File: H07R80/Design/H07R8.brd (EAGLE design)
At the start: 60 x 34.6 mm, 17 parts, among them P2 HEXABIT_X2_P1_P5_EDIT_POWER_P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, U1 STM32G0B1CEU6N, X1 XTALL_CSTCE8M00G52

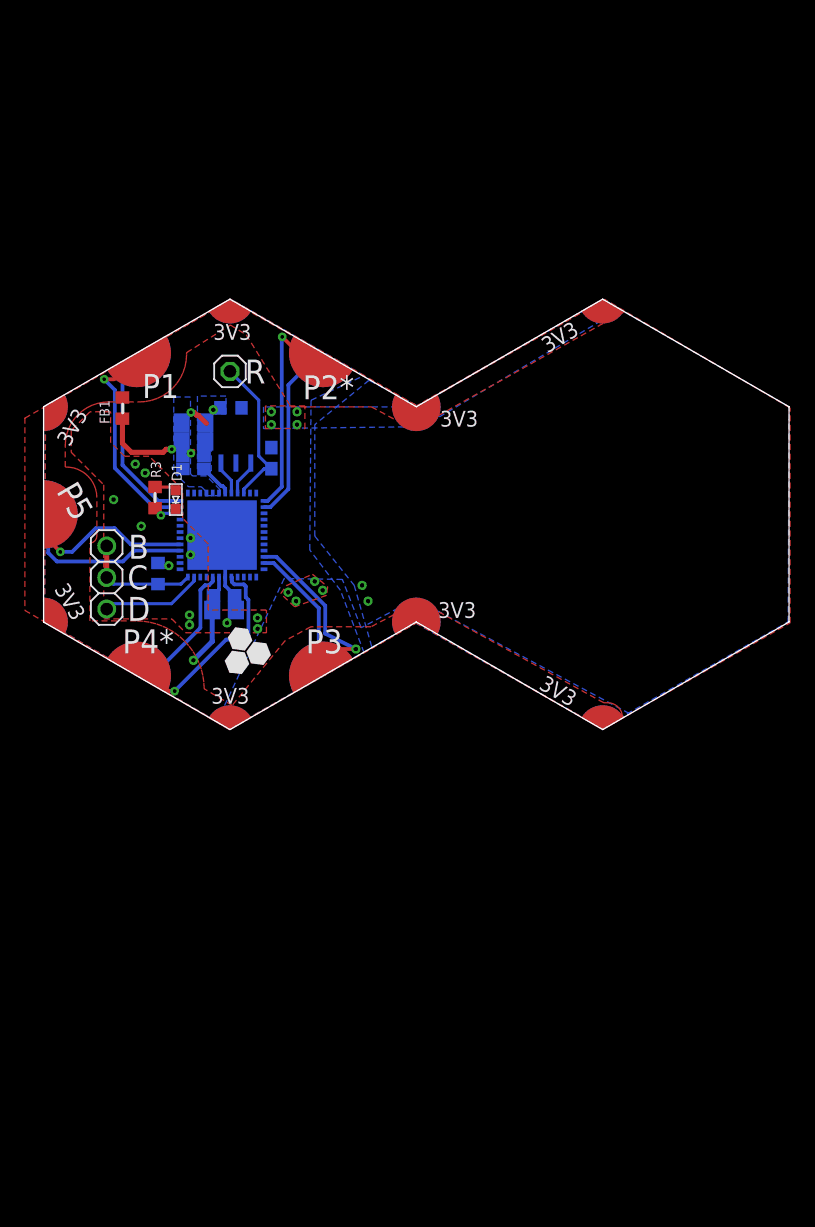
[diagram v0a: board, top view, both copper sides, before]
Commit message: - The reviewed version is complete.
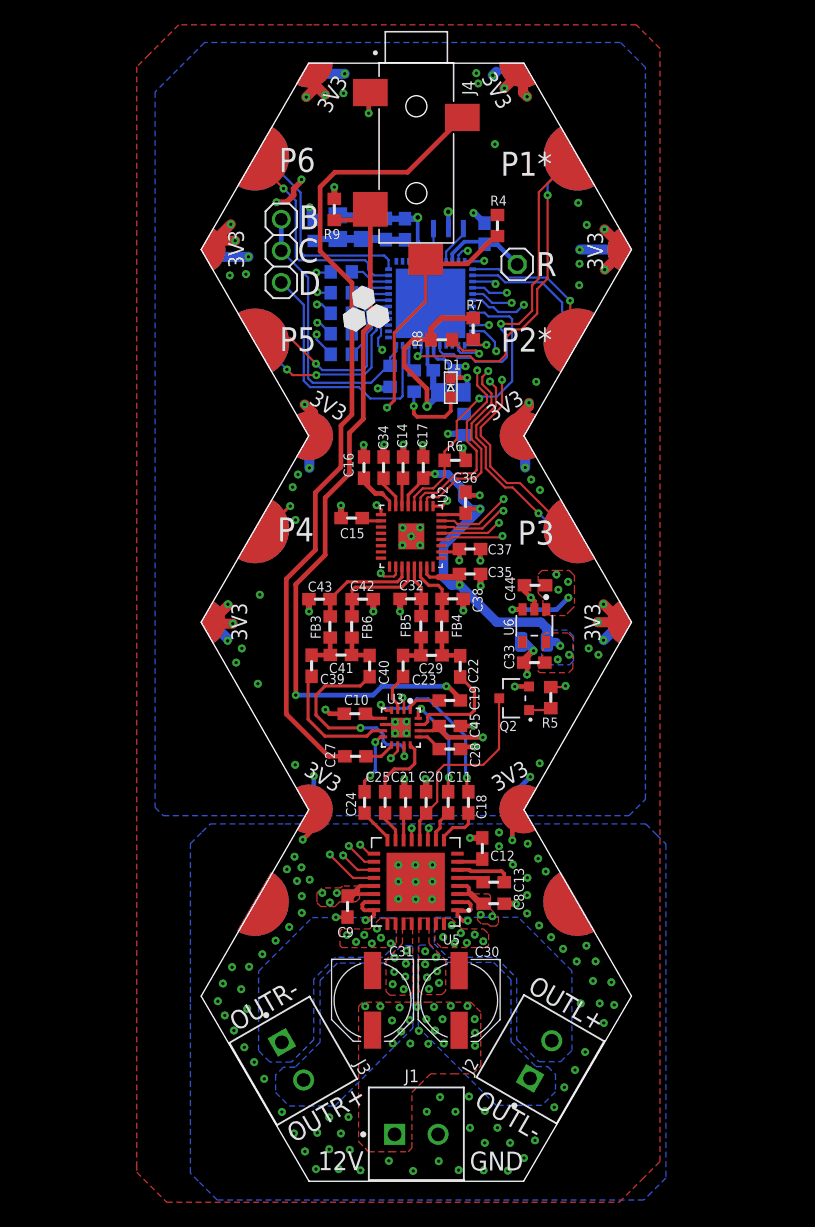
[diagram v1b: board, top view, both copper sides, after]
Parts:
- removed JP1: R, HEXABITZ_USER_INTERFACE_PARTS:1X01
- removed JP2: (no value), pinhead:1X03
- removed P2: HEXABIT_X2_P1_P5_EDIT_POWER_PADS, hexabitz_connectors:HEXABIT_X2_P1_P5_EDIT_POWER_PADS
- added +1.8V, GND: PAD4, HEXABITZ_CONNECTION_PARTS:PAD4
- added C10, C11, C18, C19, C20, C22, C23, C24, C25, C27, C28, C39, C40: 0.47uF, HEXABITZ_RCLS:C-0603
- added C12, C15, C16, C17, C33, C34, C35, C36, C37, C44: 1uF, HEXABITZ_RCLS:C-0603
- added C13, C45, C8, C9: 100nF, HEXABITZ_RCLS:C-0603
- added C14: 2.2uF, HEXABITZ_RCLS:C-0603
- added C21: 0.01uF, HEXABITZ_RCLS:C-0603
- added C29, C41: DNP, HEXABITZ_RCLS:C-0603
- added C30, C31: 47uF, HEXABITZ_RCLS:PANASONIC_D
- added C32, C38, C42, C43: 100pF, HEXABITZ_RCLS:C-0603
- added FB3, FB4, FB5, FB6: SHORT(0Ohm), HEXABITZ_RCLS:FB-0603
- added J1, J2, J3: 1751248PHOENIX_CONTACT_1751248_0_0, hexabitz_connectors:PHOENIX_CONTACT_1751248_0
- added J4: SJ-3524-SMT-TR, HEXABITZ_ICs:CUI_SJ-3524-SMT
- added P1: HEXABIT_X3_ROW_NO_P4_P6_P7_P8_P10_P14, hexabitz_connectors:HEXABIT_X3_ROW_NO_P4_P6_P7_P8_P10_P14
- added Q2: AO3400AALPHA_&_OMEGA_SEMICONDUCTOR_AO3400A_0_0, HEXABITZ_ICs:ALPHA_&_OMEGA_SEMICONDUCTOR_AO3400A_0
- added R: (no value), HEXABITZ_USER_INTERFACE_PARTS:1X01
- added R10, R11, R12, R13, R14, R5: 100, HEXABITZ_RCLS:R-0603
- added R4: 100K, HEXABITZ_RCLS:R-0603
- added R6, R9: 10K, HEXABITZ_RCLS:R-0603
- added R7, R8: 4.7K, HEXABITZ_RCLS:R-0603
- added SWD: (no value), pinhead:1X03
- added U2: MAX9867ETJ+T, HEXABITZ_ICs:QFN50P500X500X80-33N
- added U3: TS3A44159RGTRTEXAS_INSTRUMENTS_TS3A44159RGTR_0_0, HEXABITZ_ICs:TEXAS_INSTRUMENTS_TS3A44159RGTR_0
- added U5: MAX9704ETJ+, HEXABITZ_ICs:QFN65P700X700X80-33N
- added U6: MIC5365-1.8YD5-TRMICROCHIP_MIC5365-1_8YD5-TR_0_0, HEXABITZ_ICs:MICROCHIP_MIC5365-1_8YD5-TR_0
- C2: value 4.7uF -> 100nF; device HEXABITZ_RCLS:C-0805-POL -> HEXABITZ_RCLS:C-0603
- C3: value 100nF -> 4.7uF; device HEXABITZ_RCLS:C-0603 -> HEXABITZ_RCLS:C-0805-POL
- C4: value 1uF -> 100nF; device HEXABITZ_RCLS:C-0805-POL -> HEXABITZ_RCLS:C-0603
- C5: value 100nF -> 1uF; device HEXABITZ_RCLS:C-0603 -> HEXABITZ_RCLS:C-0805-POL
- D1: device Hexabitz:VLMS1300-GS08 -> HEXABITZ_USER_INTERFACE_PARTS:VLMS1300-GS08
- FB1: device HEXABITZ_RCLS:FB-0603 -> HEXABITZ_RCLS:FB-TDK_MMZ1608Y300B
- R1: value 10K -> 0.0R
- R2: value 0.0R -> 270R
- R3: value 270R -> 10K
- X1: value XTALL_CSTCE8M00G52 -> 8MHZ; device Hexabitz:XTALL_CSTCE8M00G52 -> HEXABITZ_OTHER_PARTS:XTALL_CSTCE8M00G52
- moved C5 31.7 mm to (-4.29, 31.8), turned to 90 degrees
- moved C1 29.5 mm to (5.48, 31.3), turned to 270 degrees
- moved R1 27.4 mm to (3.85, 16.0)
- moved X1 25.5 mm to (2.58, 31.7), turned to 270 degrees
- moved C7 25.3 mm to (2.78, 18.5)
- moved U1 25.1 mm to (1.14, 25.7)
- moved D1 23.9 mm to (2.77, 18.9), turned to 180 degrees
- moved C4 23.1 mm to (-0.92, 31.7), turned to 270 degrees
- moved C2 23.1 mm to (-2.45, 31.7), turned to 270 degrees
- moved C3 22.7 mm to (-6.32, 31.8), turned to 90 degrees
- moved R3 21.3 mm to (-2.11, 19.8), flipped to the bottom
- moved FB1 21.0 mm to (-8.22, 31.6), flipped to the bottom, turned to 270 degrees
- moved C6 15.6 mm to (2.21, 20.3), turned to 0 degrees
- moved R2 14.9 mm to (-0.17, 19.5), turned to 90 degrees
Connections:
- removed net CLK: JP2.1, JP2.2, R1.2, U1.36
- removed net DATA: JP2.3, U1.35
- removed net VSSA: C1.2, C2.2, C3.2, C4.2, R2.1, U1.7
- new net +1.8V: +1.8V.P$1, C17.2, C33.2, C35.2, C36.2, U2.23, U2.32, U2.5, U6.5
- new net +12V: C12.1, C30.+, C31.+, C8.1, C9.2, J1.1, U5.21, U5.22, U5.3, U5.4
- new net AUDIO_JACK_IN_L: C19.1, J4.2, R9.1
- new net AUDIO_JACK_IN_R: C27.1, J4.3
- new net C: R3.2, SWD.1, SWD.2, U1.36
- new net CODEC_IRQN_OUT: R6.1, U1.20, U2.4
- new net CODEC_LOUT_N: C32.2, FB5.1, U2.21
- new net CODEC_LOUT_P: C38.2, FB4.1, U2.22
- new net CODEC_ROUT_N: C42.2, FB6.1, U2.20
- new net CODEC_ROUT_P: C43.2, FB3.1, U2.19
- new net D: SWD.3, U1.35
- new net DC_JACK_DETECT: J4.4, R4.2, U3.10, U3.2
- new net GND1: C10.1, C14.1, C15.1, C16.1, C17.1, C2.1, C20.2, C21.2, C28.1, C3.2, C30.-, C31.-, C32.1, C33.1, C34.1, C35.1, C36.1, C37.1, C38.1, C4.1, C42.1, C43.1, C44.1, C45.2, C5.2, C8.2, C9.1, GND.P$1, J1.2, J4.1, Q2.2, R1.2, R4.1, U1.7, U2.1, U2.18, U2.33, U2.9, U3.17, U3.6, U5.1, U5.13, U5.2, U5.23, U5.24, U5.33, U6.2
- new net I2C_SCL: R7.2, U1.25, U2.2
- new net I2C_SDA: R8.2, U1.26, U2.3
- new net I2S_CLK: U1.16, U2.30
- new net I2S_MCK: U1.17, U2.31
- new net I2S_SD: U1.18, U2.28
- new net I2S_WS: U1.15, U2.29
- new net N$10: C13.1, U5.6
- new net N$11: C39.2, U3.7
- new net N$12: C1.2, R.1, U1.10
- new net N$13: C40.2, U3.11
- new net N$14: C19.2, U3.1
- new net N$15: C13.2, U5.5
- new net N$17: C27.2, U3.9
- new net N$18: C22.1, C29.2, FB4.2
- new net N$19: C23.1, C29.1, FB5.2
- new net N$20: C39.1, C41.2, FB3.2
- new net N$21: C10.2, U3.5
- new net N$22: C28.2, U3.13
- new net N$23: C16.2, U2.8
- new net N$24: C14.2, U2.6
- new net N$25: C34.2, U2.7
- new net N$26: C11.2, U5.10
- new net N$27: C11.1, U3.16
- new net N$28: C18.1, U3.4
- new net N$29: C24.1, U3.8
- new net N$3: R2.2, U1.34
- new net N$30: C25.1, U3.12
- new net N$33: C18.2, U5.9
- new net N$34: C24.2, U5.16
- new net N$35: C15.2, U2.10
- new net N$36: C20.1, Q2.3, U5.12
- new net N$37: C25.2, U5.15
- new net N$39: R13.1, U5.19
- new net N$4: D1.A, R2.1
- new net N$40: R14.1, U5.20
- new net N$41: R12.1, U5.11
- new net N$42: R11.1, U5.17
- new net N$43: R10.1, U5.18
- new net N$44: Q2.1, R5.1
- new net N$45: U1.33
- new net N$7: C12.2, U5.7
- new net N$9: C23.2, U3.3
- new net OUTL+: J2.2, U5.31, U5.32
- new net OUTL-: J2.1, U5.29, U5.30
- new net OUTR+: J3.2, U5.27, U5.28
- new net OUTR-: J3.1, U5.25, U5.26
- new net PWR_AMP_FSEL1: R13.2, U1.43
- new net PWR_AMP_FSEL2: R14.2, U1.42
- new net PWR_AMP_GAIN1: R11.2, U1.45
- new net PWR_AMP_GAIN2: R10.2, U1.44
- new net PWR_AMP_MUTE: R5.2, U1.39
- new net PWR_AMP_SHDN: R12.2, U1.46
- new net USART4_RX: P1.PAD_PD11, U1.12
- new net USART4_TX: P1.PAD_PU11, U1.11
- net GND: now also C1.1, C6.1, P1.PAD_PD15, P1.PAD_PD16, P1.PAD_PD17, P1.PAD_PD18, P1.PAD_PD19, P1.PAD_PD24, P1.PAD_PD25, P1.PAD_PD26, P1.PAD_PD27, P1.PAD_PD28, R3.1; no longer C5.2, C6.2, P2.PAD_PD11, P2.PAD_PD12, P2.PAD_PD13, P2.PAD_PD14, P2.PAD_PD17, P2.PAD_PD18, P2.PAD_PD19, P2.PAD_PD20, R2.2
- net N$1: now also U1.8, X1.P$1; no longer D1.A, R3.2
- net N$2: now also U1.9, X1.P$3; no longer R3.1, U1.46
- net N$5: now also C40.1, C41.1, FB6.2; no longer U1.9, X1.P$1
- net N$6: now also C21.1, U5.14; no longer U1.8, X1.P$3
- net N$8: now also C22.2, U3.15; no longer C6.1, JP1.1, U1.10
- net USART1_RX: now also P1.PAD_PD1; no longer P2.PAD_PD4
- net USART1_TX: now also P1.PAD_PU1; no longer P2.PAD_PU4
- net USART2_RX: now also P1.PAD_PD2; no longer P2.PAD_PD2
- net USART2_TX: now also P1.PAD_PU2; no longer P2.PAD_PU2
- net USART3_RX: now also P1.PAD_PD3; no longer P2.PAD_PD3
- net USART3_TX: now also P1.PAD_PU3; no longer P2.PAD_PU3
- net USART5_RX: now also P1.PAD_PD12; no longer P2.PAD_PD5
- net USART5_TX: now also P1.PAD_PU12; no longer P2.PAD_PU5
- net USART6_RX: now also P1.PAD_PD13; no longer P2.PAD_PD1
- net USART6_TX: now also P1.PAD_PU13; no longer P2.PAD_PU1
- net VDD: now also C37.2, C44.2, C45.1, C6.2, FB1.1, P1.PAD_PU15, P1.PAD_PU16, P1.PAD_PU17, P1.PAD_PU18, P1.PAD_PU19, P1.PAD_PU24, P1.PAD_PU25, P1.PAD_PU26, P1.PAD_PU27, P1.PAD_PU28, R6.2, R7.1, R8.1, R9.2, U2.26, U3.14, U6.1, U6.3; no longer C5.1, FB1.2, P2.PAD_PU11, P2.PAD_PU12, P2.PAD_PU13, P2.PAD_PU14, P2.PAD_PU17, P2.PAD_PU18, P2.PAD_PU19, P2.PAD_PU20
- net VDDA: now also C2.2, C4.2, C5.1, FB1.2; no longer C1.1, C2.1, C4.1, FB1.1
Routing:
- net AUDIO_JACK_IN_R: track 0.00 -> 65.6 mm
- net VDD: track 7.70 -> 71.7 mm, vias 1 -> 27
- net AUDIO_JACK_IN_L: track 0.00 -> 58.9 mm, vias 0 -> 2
- net GND1: track 0.00 -> 58.1 mm, vias 0 -> 144
- net DC_JACK_DETECT: track 0.00 -> 54.6 mm, vias 0 -> 3
- net N$41: track 0.00 -> 51.4 mm, vias 0 -> 2
- net N$40: track 0.00 -> 50.5 mm, vias 0 -> 2
- net N$43: track 0.00 -> 50.2 mm, vias 0 -> 2
- net N$39: track 0.00 -> 50.1 mm, vias 0 -> 2
- net N$42: track 0.00 -> 49.8 mm, vias 0 -> 2
- net USART4_RX: track 0.00 -> 41.5 mm, vias 0 -> 2
- net USART4_TX: track 0.00 -> 39.7 mm, vias 0 -> 2
- net PWR_AMP_MUTE: track 0.00 -> 39.1 mm, vias 0 -> 2
- net GND: track 6.49 -> 45.3 mm, vias 20 -> 21
- net +1.8V: track 0.00 -> 35.8 mm, vias 0 -> 6
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- added copper zone on layer 1, net +1.8V
- added copper zone on layer 16, net +1.8V
- added copper zone on layer 1, net +12V
- added copper zone on layer 15, net +12V
- added copper zone on layer 2, net GND
- added copper zone on layer 1, net GND1
- added copper zone on layer 16, net GND1
- added copper zone on layer 2, net GND1
- added copper zone on layer 1, net OUTL+
- added copper zone on layer 16, net OUTL+
- added copper zone on layer 1, net OUTL-
- added copper zone on layer 16, net OUTL-
- added copper zone on layer 1, net OUTR+
- added copper zone on layer 16, net OUTR+
- added copper zone on layer 1, net OUTR-
- added copper zone on layer 16, net OUTR-
- added copper zone on layer 15, net VDD
- removed copper zone on layer 1, net GND
- removed copper zone on layer 16, net VDDA
- removed copper zone on layer 1, net VSSA
- removed copper zone on layer 16, net VSSA
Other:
- board size 60 x 34.6 mm -> 34.6 x 90 mm
- board text added: "10W"
- board text added: "12V"
- board text added: "OUTL+"
- board text added: "OUTL-"
- board text added: "OUTR+"
- board text added: "OUTR-"
- board text added: "P1*"
- board text added: "P4"
- board text added: "P6"
- board text removed: "P1"
- board text removed: "P4*"
